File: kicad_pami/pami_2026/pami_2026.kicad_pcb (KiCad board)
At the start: 4 copper layers, 50 x 80 mm, 61 parts, among them J1 Conn_01x04_Socket, J10 Conn_01x07_Socket, J11 Conn_01x06, J12 Conn_01x06, J14 Conn_01x03_Pin, J2 Conn_01x03_Pin, J3 Conn_01x04_Pin, J4 Conn_01x02_Pin, J7 Conn_01x03_Pin, J8 USB_C_Receptacle_USB2.0_14P, J9 Conn_01x04_Pin, Q1 NMOS, Q2 NMOS, Q3 NMOS, SW1 SW_Push, SW2 SW_DIP_x01, SW3 SW_Push_Open, SW4 SW_Reed, U1 DRV8833RTY, U2 ESP32-S3-MINI-1, U3 LD1117S33TR_SOT223, U4 L7805

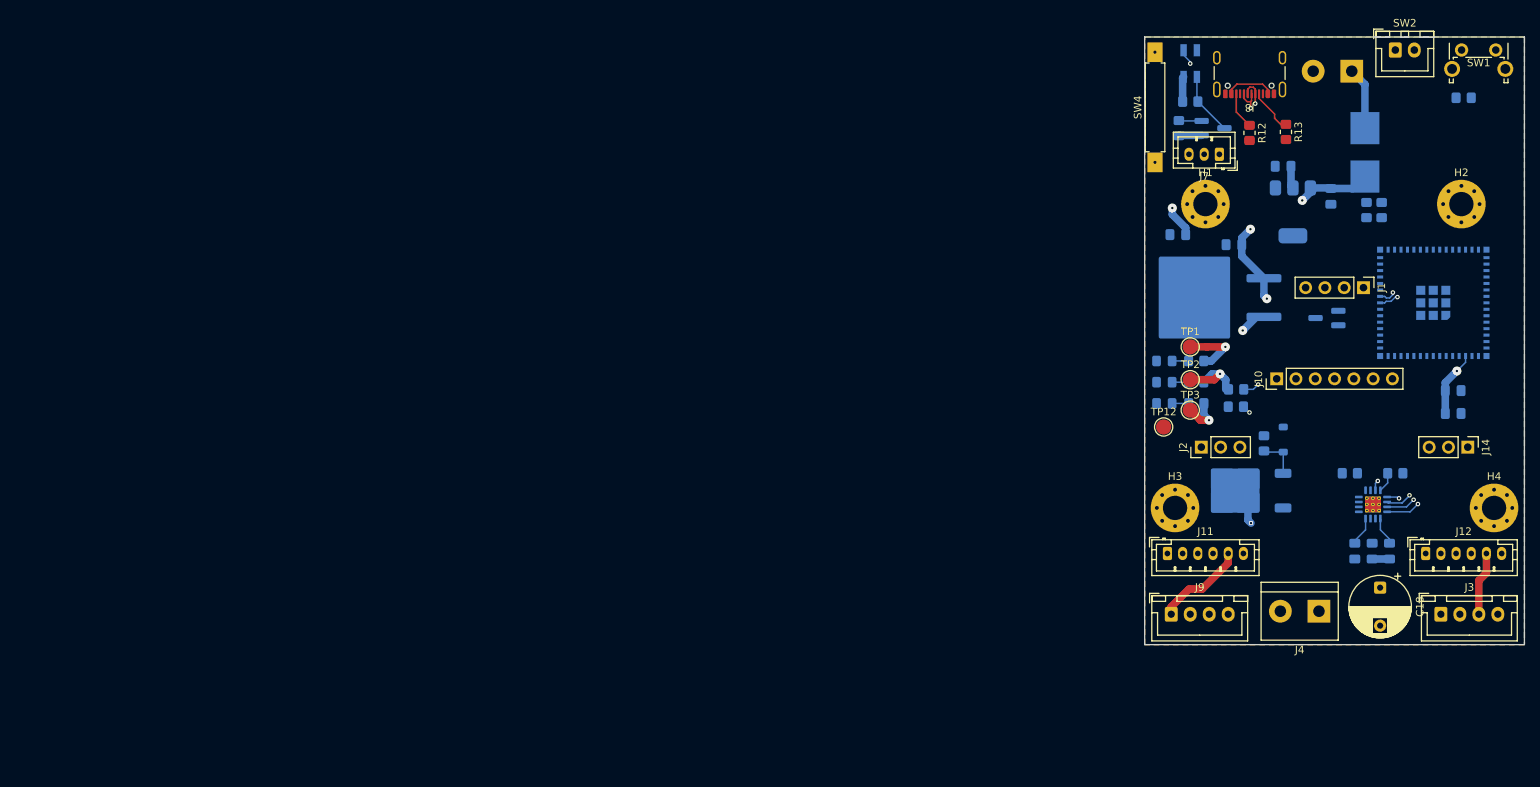
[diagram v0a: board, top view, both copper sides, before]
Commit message: ajout code / avancement pcb et 3D
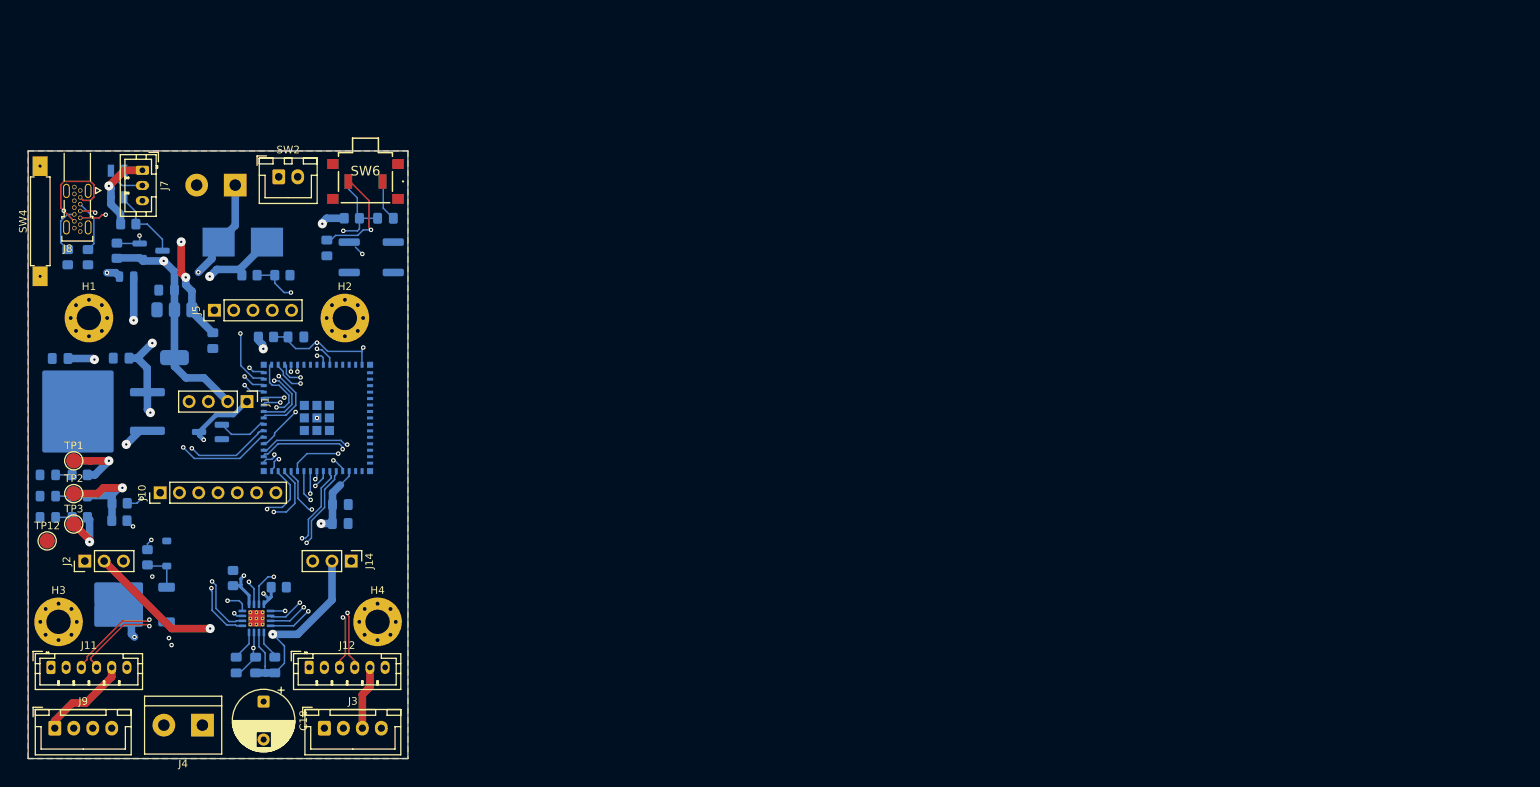
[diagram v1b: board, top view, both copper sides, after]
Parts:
- removed C24: 4.7u, Capacitor_SMD:C_0805_2012Metric_Pad1.18x1.45mm_HandSolder
- added C4: 100n, Capacitor_SMD:C_0805_2012Metric_Pad1.18x1.45mm_HandSolder, B.Cu at (82.1, 90.1)
- added C5: 100n, Capacitor_SMD:C_0805_2012Metric_Pad1.18x1.45mm_HandSolder, B.Cu at (88.0, 49.9)
- added C6: 100n, Capacitor_SMD:C_0805_2012Metric_Pad1.18x1.45mm_HandSolder, B.Cu at (76.3, 65.5)
- added C7: 100n, Capacitor_SMD:C_0805_2012Metric_Pad1.18x1.45mm_HandSolder, B.Cu at (80.3, 53.8)
- added D1: D, Diode_SMD:D_0805_2012Metric, B.Cu at (54.0, 57.5)
- added J5: Conn_01x05_Pin, Connector_PinHeader_2.54mm:PinHeader_1x05_P2.54mm_Vertical, F.Cu at (65.5, 62.0)
- added R14: R, Resistor_SMD:R_0805_2012Metric_Pad1.20x1.40mm_HandSolder, B.Cu at (83.6, 49.9)
- added SW5: SW_Push, CustomLibrary:PTS645VSM19PSMTR92LFS, B.Cu at (85.4, 44.5)
- added SW6: SW_Push, CustomLibrary:PTS645VSM19PSMTR92LFS, F.Cu at (85.4, 44.5)
- J8: footprint Connector_USB:USB_C_Receptacle_GCT_USB4105-xx-A_16P_TopMnt_Horizontal -> CustomLibrary:MOLEX_2169890001
- R12, R13: moved to B.Cu
- SW1: footprint Button_Switch_THT:SW_Tactile_SPST_Angled_PTS645Vx39-2LFS -> Button_Switch_SMD:SW_Push_1P1T_NO_CK_KSC9xxJ; moved to B.Cu
- U2: footprint RF_Module:ESP32-S2-MINI-1 -> CustomLibrary:ESP32S3MINI1N8
- moved R1 160.8 mm to (72.3, 65.5)
- moved R13 158.6 mm to (48.9, 55.0)
- moved R12 156.5 mm to (46.2, 55.0)
- moved J8 154.8 mm to (47.5, 41.2)
- moved U2 150.3 mm to (79.0, 76.2)
- moved R17 149.3 mm to (70.1, 57.4), turned to 180 degrees
- moved C9 148.4 mm to (65.3, 66.0)
- moved F1 148.2 mm to (69.3, 53.0), turned to 0 degrees
- moved U3 148.1 mm to (60.3, 65.1)
- moved C12 148.1 mm to (45.2, 68.3)
- moved C1 148.0 mm to (68.4, 108.7)
- moved SW2 148.0 mm to (74.0, 44.4)
- moved C10 147.9 mm to (59.2, 59.3)
- moved C18 147.8 mm to (72.0, 113.5)
- moved C2 147.8 mm to (70.9, 108.7)
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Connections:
- net Net-(U2-EN) renamed EN
- C9 pad 1: +BATT -> +5V
- J10 pad 5: tft_scl -> tft_sda
- U2 pad 10: unconnected-(U2-IO6-Pad10) -> motor_b_sense
- U2 pad 11: unconnected-(U2-IO7-Pad11) -> motor_fault
- U2 pad 12: unconnected-(U2-IO8-Pad12) -> SERVO2
- U2 pad 13: unconnected-(U2-IO9-Pad13) -> SERVO1
- U2 pad 14: unconnected-(U2-IO10-Pad14) -> motor_enable
- U2 pad 15: unconnected-(U2-IO11-Pad15) -> motor_a+
- U2 pad 16: unconnected-(U2-IO12-Pad16) -> motor_a-
- U2 pad 17: unconnected-(U2-IO13-Pad17) -> motor_b+
- U2 pad 18: unconnected-(U2-IO14-Pad18) -> motor_b-
- U2 pad 19: unconnected-(U2-IO15-Pad19) -> LEVEL_BATTERY
- U2 pad 20: unconnected-(U2-IO16-Pad20) -> I2C_scl
- U2 pad 21: unconnected-(U2-IO17-Pad21) -> I2C_sda
- U2 pad 22: unconnected-(U2-IO18-Pad22) -> EN_SCREEN
- U2 pad 25: unconnected-(U2-IO21-Pad25) -> RX_lidar
- U2 pad 26: unconnected-(U2-IO26-Pad26) -> TX_lidar
- U2 pad 27: unconnected-(U2-IO47-Pad27) -> sw_team
- U2 pad 28: unconnected-(U2-IO33-Pad28) -> button_user
- U2 pad 29: unconnected-(U2-IO34-Pad29) -> NEOPIXEL
- U2 pad 30: unconnected-(U2-IO48-Pad30) -> sw_tirette
- U2 pad 31: unconnected-(U2-IO35-Pad31) -> tft_sda
- U2 pad 32: unconnected-(U2-IO36-Pad32) -> tft_scl
- U2 pad 33: unconnected-(U2-IO37-Pad33) -> tft_dc
- U2 pad 34: unconnected-(U2-IO38-Pad34) -> tft_rst
- U2 pad 35: unconnected-(U2-IO39-Pad35) -> tft_cs
- U2 pad 39: unconnected-(U2-TXD0-Pad39) -> TX0
- U2 pad 4: unconnected-(U2-IO0-Pad4) -> GPIO0
- U2 pad 40: unconnected-(U2-RXD0-Pad40) -> RX0
- U2 pad 5: unconnected-(U2-IO1-Pad5) -> motor_enc_b-
- U2 pad 6: unconnected-(U2-IO2-Pad6) -> motor_enc_b+
- U2 pad 7: unconnected-(U2-IO3-Pad7) -> motor_enc_a-
- U2 pad 8: unconnected-(U2-IO4-Pad8) -> motor_enc_a+
- U2 pad 9: unconnected-(U2-IO5-Pad9) -> motor_a_sense
- U3 pad 3: +BATT -> +5V
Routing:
- net Net-(J4-Pin_1): track 0.00 -> 99.5 mm
- net +5V: track 69.0 -> 161.1 mm, vias 3 -> 9
- net +3.3V: track 159.6 -> 220.0 mm, vias 2 -> 5
- net GPIO0: track 0.00 -> 56.6 mm, vias 0 -> 2
- net TX_lidar: track 0.00 -> 55.4 mm, vias 0 -> 1
- net Net-(SW3-A): track 8.22 -> 61.8 mm, vias 0 -> 2
- net RX_lidar: track 0.00 -> 53.5 mm, vias 0 -> 1
- net +BATT: track 47.5 -> 93.6 mm
- net button_user: track 0.00 -> 46.1 mm, vias 0 -> 2
- net motor_enc_a-: track 0.00 -> 44.9 mm, vias 0 -> 2
- net motor_enc_a+: track 0.00 -> 44.5 mm, vias 0 -> 2
- net sw_team: track 0.00 -> 42.2 mm, vias 0 -> 1
- net EN: track 0.00 -> 37.6 mm, vias 0 -> 3
- net sw_tirette: track 0.00 -> 35.6 mm, vias 0 -> 1
- net motor_a-: track 0.00 -> 33.3 mm, vias 0 -> 2
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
